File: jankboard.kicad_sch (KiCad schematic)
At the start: 157 parts, among them J1 F31L-1A7H1-11030, J2 F31L-1A7H1-11030, J3 Conn_01x02, J4 Conn_01x02, J5 Conn_01x04_Pin, SW1 SW_Push_45deg, SW10 SW_Push_45deg, SW11 SW_Push_45deg, SW12 SW_Push_45deg, SW13 SW_Push_45deg, SW14 SW_Push_45deg, SW15 SW_Push_45deg, SW16 SW_Push_45deg, SW17 SW_Push_45deg, SW18 SW_Push_45deg, SW19 SW_Push_45deg, SW2 SW_Push_45deg, SW20 SW_Push_45deg, SW21 SW_Push_45deg, SW3 SW_Push_45deg, SW4 SW_Push_45deg, SW5 SW_Push_45deg, SW6 SW_Push_45deg, SW7 SW_Push_45deg, SW8 SW_Push_45deg, SW9 SW_Push_45deg, U1 nice_nano

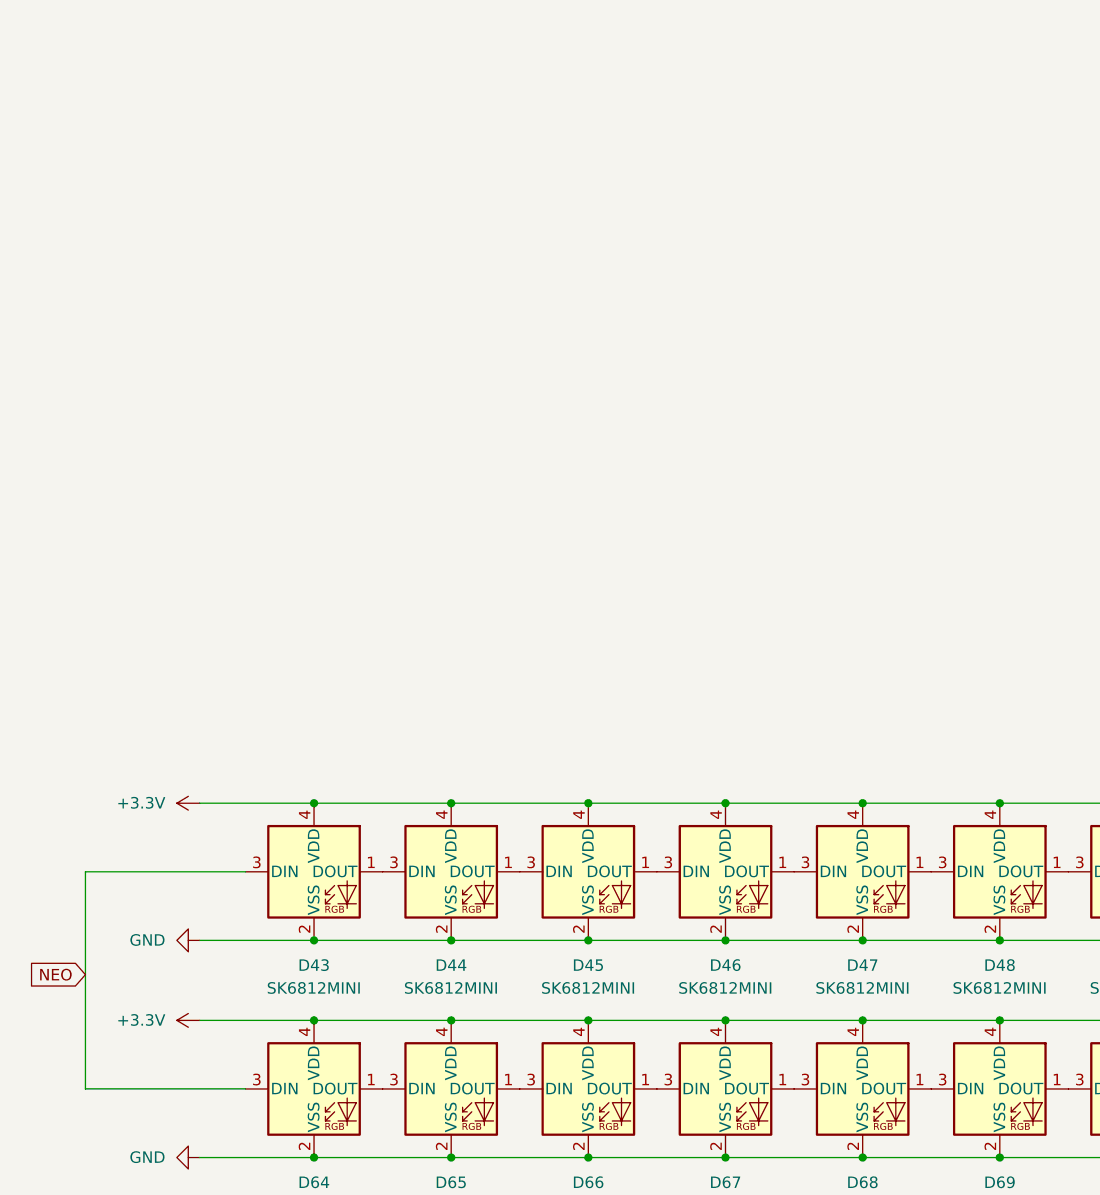
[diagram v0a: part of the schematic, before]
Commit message: add led switch
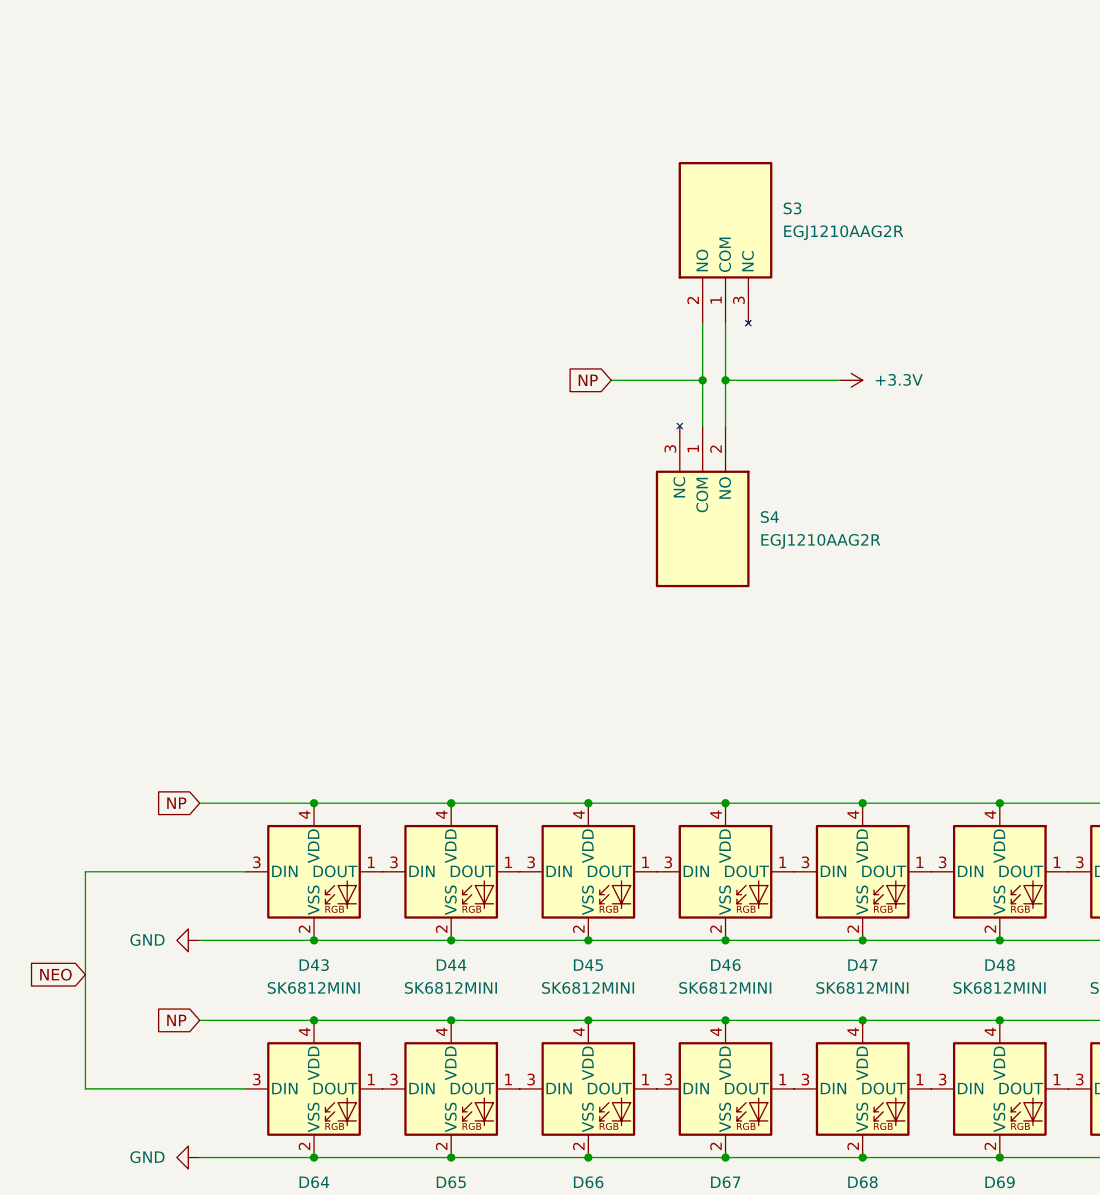
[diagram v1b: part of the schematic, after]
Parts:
- added S3, S4: EGJ1210AAG2R, KiCad:EGJ1210AAG2R, symbol EGJ1210AAG2R:EGJ1210AAG2R
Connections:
- net +3.3V: now also S3.1 (COM), S4.2 (NO); no longer D43.4 (VDD), D44.4 (VDD), D45.4 (VDD), D46.4 (VDD), D47.4 (VDD), D48.4 (VDD), D49.4 (VDD), D50.4 (VDD), D51.4 (VDD), D52.4 (VDD), D53.4 (VDD), D54.4 (VDD), D55.4 (VDD), D56.4 (VDD), D57.4 (VDD), D58.4 (VDD), D59.4 (VDD), D60.4 (VDD), D61.4 (VDD), D62.4 (VDD), D63.4 (VDD), D64.4 (VDD), D65.4 (VDD), D66.4 (VDD), D67.4 (VDD), D68.4 (VDD), D69.4 (VDD), D70.4 (VDD), D71.4 (VDD), D72.4 (VDD), D73.4 (VDD), D74.4 (VDD), D75.4 (VDD), D76.4 (VDD), D77.4 (VDD), D78.4 (VDD), D79.4 (VDD), D80.4 (VDD), D81.4 (VDD), D82.4 (VDD), D83.4 (VDD), D84.4 (VDD)
- new net NP: D43.4 (VDD), D44.4 (VDD), D45.4 (VDD), D46.4 (VDD), D47.4 (VDD), D48.4 (VDD), D49.4 (VDD), D50.4 (VDD), D51.4 (VDD), D52.4 (VDD), D53.4 (VDD), D54.4 (VDD), D55.4 (VDD), D56.4 (VDD), D57.4 (VDD), D58.4 (VDD), D59.4 (VDD), D60.4 (VDD), D61.4 (VDD), D62.4 (VDD), D63.4 (VDD), D64.4 (VDD), D65.4 (VDD), D66.4 (VDD), D67.4 (VDD), D68.4 (VDD), D69.4 (VDD), D70.4 (VDD), D71.4 (VDD), D72.4 (VDD), D73.4 (VDD), D74.4 (VDD), D75.4 (VDD), D76.4 (VDD), D77.4 (VDD), D78.4 (VDD), D79.4 (VDD), D80.4 (VDD), D81.4 (VDD), D82.4 (VDD), D83.4 (VDD), D84.4 (VDD), S3.2 (NO), S4.1 (COM)
